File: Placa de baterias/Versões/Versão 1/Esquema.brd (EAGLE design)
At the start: 41.9 x 28.6 mm, 7 parts

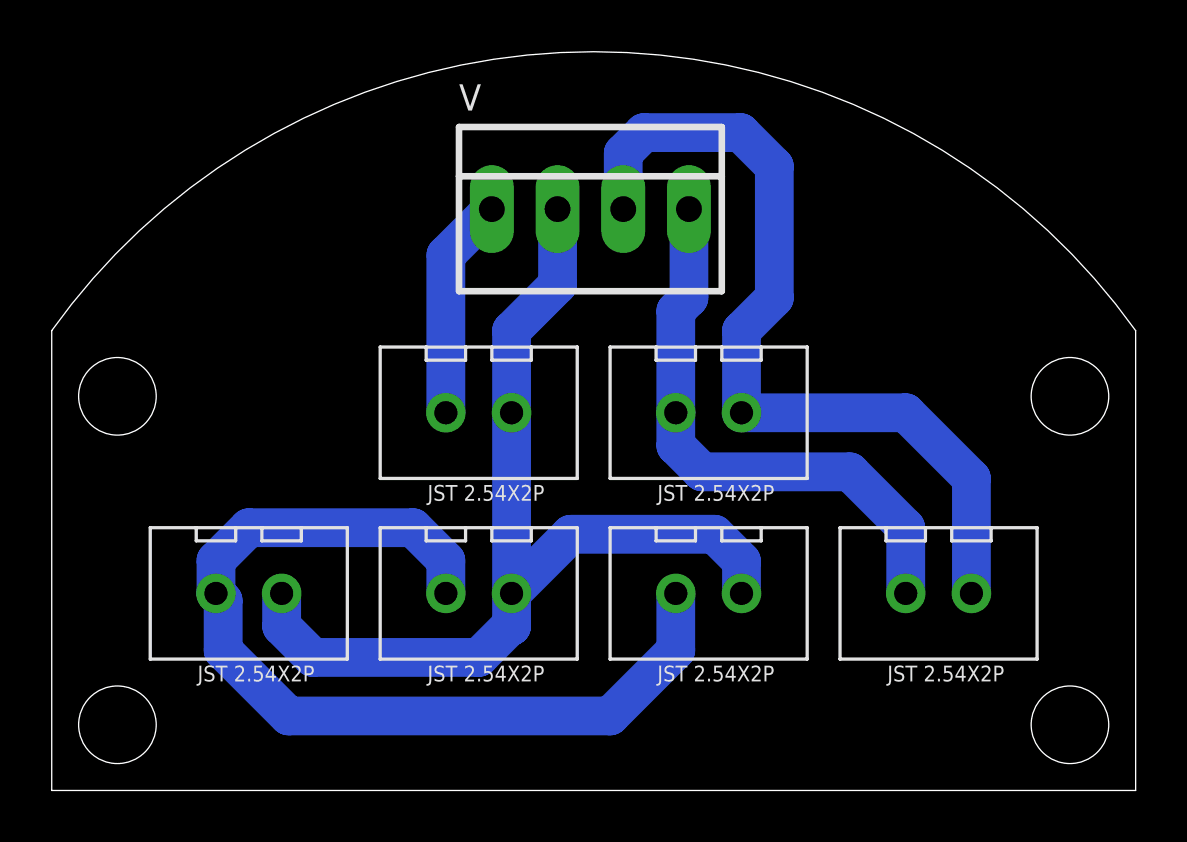
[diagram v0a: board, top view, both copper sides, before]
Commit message: teste
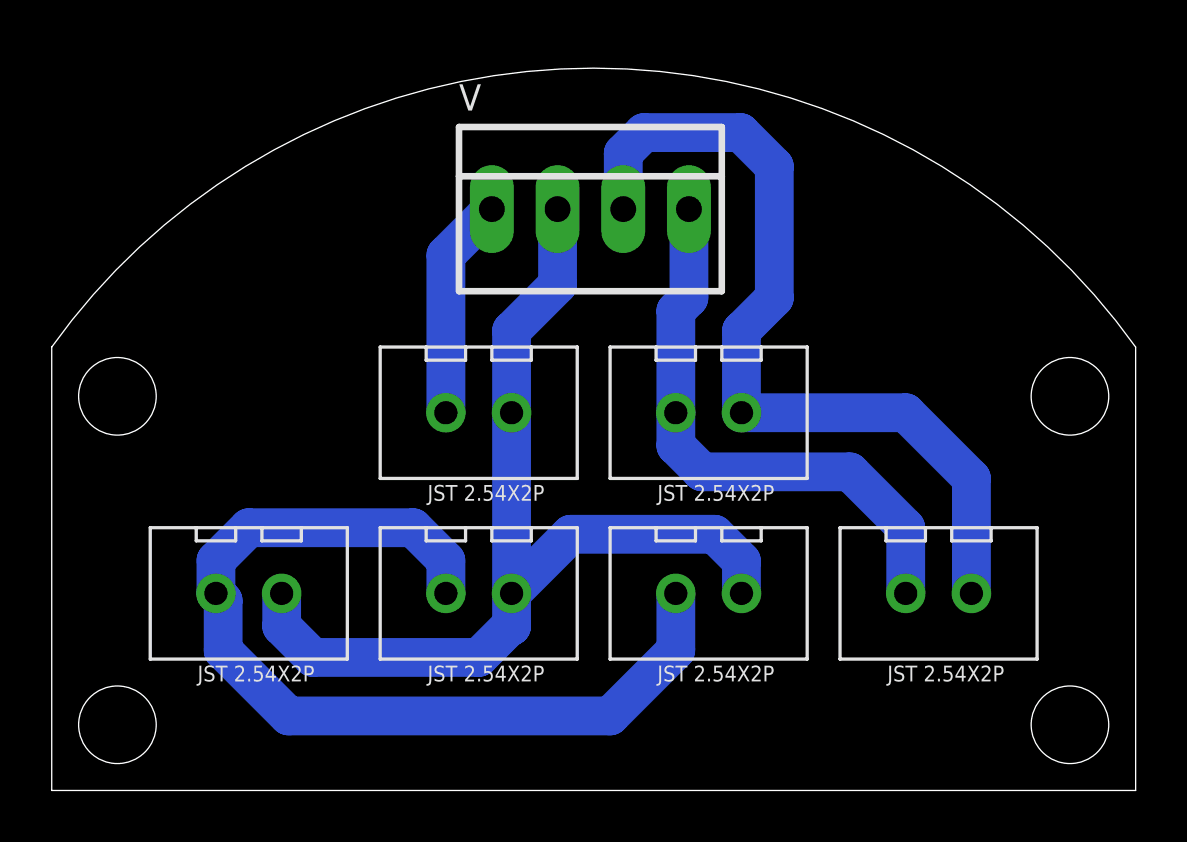
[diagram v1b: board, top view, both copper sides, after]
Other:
- board size 41.9 x 28.6 mm -> 41.9 x 27.9 mm
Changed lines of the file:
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@@
 </layers>
 <board>
-<fusionsync huburn="a.YnVzaW5lc3M6ZGlzY2VudGUxNzg" projecturn="a.YnVzaW5lc3M6ZGlzY2VudGUxNzgjRDIwMjIwNjExNTMyNjQzNTAx" f3durn="urn:adsk.wipprod:dm.lineage:PkS-i6vOSt6JP8FzX6P3mg" pcbguid="" lastpulledtime="" lastsyncedchangeguid="" latestrevisionid="dae5b02e-3f86-4753-98fb-deca12bab6cc" lastsyncedrevisionid="dae5b02e-3f86-4753-98fb-deca12bab6cc" lastboardhashguid="e1b1cba6-bc9d-dcd1-c240-c72e3c8944e4" lastpushedtime="2025-07-01T22:19:30Z" linktopcb3d="true"/>
+<fusionsync huburn="a.YnVzaW5lc3M6ZGlzY2VudGUxNzg" projecturn="a.YnVzaW5lc3M6ZGlzY2VudGUxNzgjRDIwMjIwNjExNTMyNjQzNTAx" f3durn="urn:adsk.wipprod:dm.lineage:Dvtrc6K0SWqyUMVJzSpTWQ" pcbguid="" lastpulledtime="" lastsyncedchangeguid="" latestrevisionid="de83ba8c-14a2-4f2c-87d4-37bcf2589fd9" lastsyncedrevisionid="de83ba8c-14a2-4f2c-87d4-37bcf2589fd9" lastboardhashguid="3ac31985-926d-b8f2-58d9-c6a5415b0390" lastpushedtime="2025-09-09T18:21:38Z" linktopcb3d="true"/>
 <plain>
 <hole x="39.37" y="15.24" drill="3"/>
@@
 <hole x="2.54" y="2.54" drill="3"/>
 <hole x="2.54" y="15.24" drill="3"/>
-<wire x1="41.91" y1="0" x2="41.91" y2="17.78" width="0" layer="20"/>
-<wire x1="0" y1="17.78" x2="41.91" y2="17.78" width="0" layer="20" curve="-108.924644"/>
-<wire x1="0" y1="17.78" x2="0" y2="0" width="0" layer="20"/>
+<wire x1="41.91" y1="0" x2="41.91" y2="17.145" width="0" layer="20"/>
+<wire x1="0" y1="17.145" x2="41.91" y2="17.145" width="0" layer="20" curve="-108.924644"/>
+<wire x1="0" y1="17.145" x2="0" y2="0" width="0" layer="20"/>
 <wire x1="0" y1="0" x2="41.91" y2="0" width="0" layer="20"/>
 <dimension x1="0" y1="-1.27" x2="41.91" y2="-1.27" x3="20.955" y3="-3.81" textsize="1.778" layer="27"/>
